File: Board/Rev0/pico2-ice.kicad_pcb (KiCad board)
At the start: 4 copper layers, 22.9 x 61 mm, 101 parts, among them J1 USB_C_Receptacle_USB2.0, J2 Conn_02x20_Odd_Even, J3 Conn_02x20_Odd_Even, J4 PB_SEL, Q1 2N7002, SW1 PTS820 J25K SMTR LFS, SW2 PTS820 J25K SMTR LFS, U1 NCP115AMX120TCG, U2 W25Q32JVSSIQ, U3 RP2040, U4 NCP115AMX330TCG, U5 APS6404L-3SQN-SN, U6 ICE40UP5K-SG48ITR, U8 W25Q32JVSSIQ, Y1 12 MHz

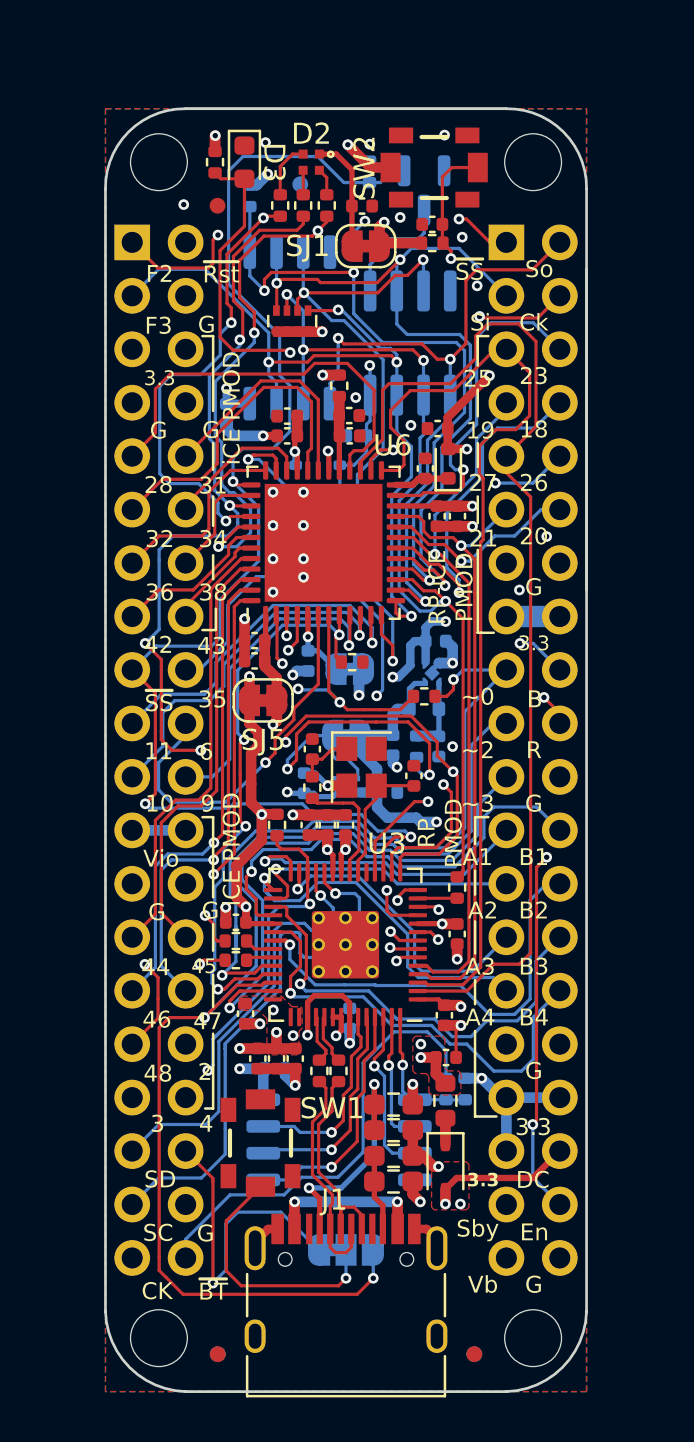
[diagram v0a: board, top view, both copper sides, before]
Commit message: Complete the layout for a review.
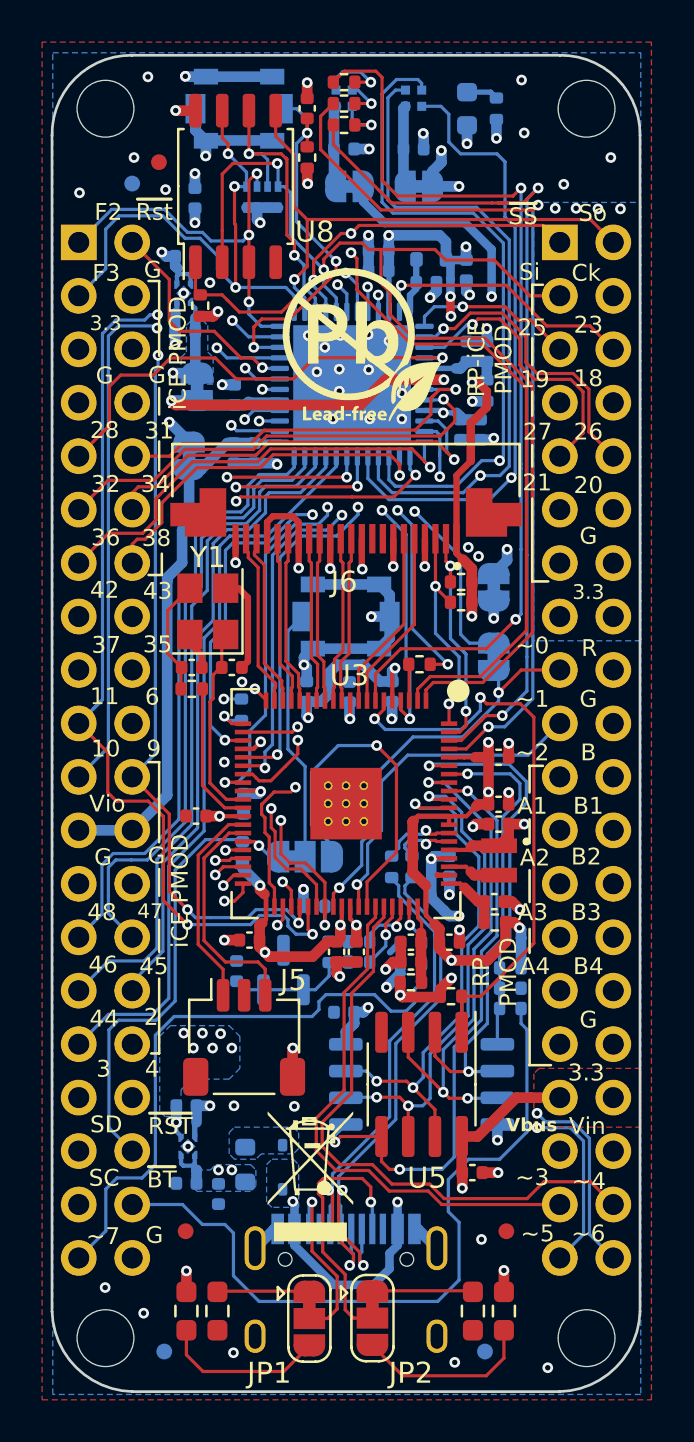
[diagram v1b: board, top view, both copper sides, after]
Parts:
- removed D6: 1N4148WT-7, Diode_SMD:D_SOD-523
- removed Q1: 2N7002, Package_TO_SOT_SMD:SOT-23
- added C20: 4.7u, Capacitor_SMD:C_0402_1005Metric, B.Cu at (77.3, 109.7)
- added C23: 4.7u, Capacitor_SMD:C_0402_1005Metric, F.Cu at (79.4, 111.3)
- added C35: 4.7u, Capacitor_SMD:C_0402_1005Metric, F.Cu at (75.5, 114.2)
- added C38: 4.7u, Capacitor_SMD:C_0402_1005Metric, F.Cu at (79.6, 107.7)
- added C39: 4.7u, Capacitor_SMD:C_0402_1005Metric, B.Cu at (64.8, 124.7)
- added C41: 4.7u, Capacitor_SMD:C_0402_1005Metric, B.Cu at (64.8, 121.0)
- added J5: SM03B-SRSS-TB, Connector_JST:JST_SH_SM03B-SRSS-TB_1x03-1MP_P1.00mm_Horizontal, F.Cu at (67.5, 117.8)
- added J6: Conn_01x22_MountingPin, RP2350_60QFN_minimal:AMPHENOL_SFV22R-2STE1HLF, F.Cu at (72.4, 91.7)
- added JP1: SolderJumper_3_Bridged12, Jumper:SolderJumper-3_P1.3mm_Bridged12_RoundedPad1.0x1.5mm, F.Cu at (70.6, 131.1)
- added JP2: SolderJumper_3_Bridged12, Jumper:SolderJumper-3_P1.3mm_Bridged12_RoundedPad1.0x1.5mm, F.Cu at (73.6, 131.1)
- added L1: 3.3u, RP2350_60QFN_minimal:L_pol_2016, F.Cu at (79.7, 109.4)
- added R26: 27, Resistor_SMD:R_0402_1005Metric, F.Cu at (79.5, 112.3)
- added R27: DNF, Resistor_SMD:R_0402_1005Metric, B.Cu at (80.2, 115.5)
- added R28: 10K, Resistor_SMD:R_0402_1005Metric, B.Cu at (75.5, 113.3)
- added R29: 10K, Resistor_SMD:R_0402_1005Metric, B.Cu at (75.5, 114.3)
- added R30: 0, Resistor_SMD:R_0402_1005Metric, B.Cu at (73.0, 114.2)
- added R31: 0, Resistor_SMD:R_0402_1005Metric, B.Cu at (73.0, 113.2)
- added SJ3: SHORT, Jumper:SolderJumper-2_P1.3mm_Bridged_RoundedPad1.0x1.5mm, B.Cu at (79.4, 99.7)
- added SJ6: SHORT, Jumper:SolderJumper-2_P1.3mm_Bridged_RoundedPad1.0x1.5mm, B.Cu at (79.4, 96.4)
- added U9: NCP115AMX330TCG, RP2040_minimal:OnSemi_XDFN4-1EP_1.0x1.0mm_EP0.52x0.52mm, B.Cu at (64.9, 123.0)
- C1, C2: value 27p -> 15p
- C15, C16, C17, C21, C22, C24, C25, C28, C29, C3, C30, C31, C32, C33, C34, C6, D1, D2, D3, D5, J1, PTC1, R11, R14, R16, R4, R5, R7, RN1, SJ1, SJ5, SW1, SW2, U6: moved to B.Cu
- C4, C42, LOGO2, LOGO3, R13, R8, U5, U8: moved to F.Cu
- C9: value 4.7u -> 0.1u; moved to F.Cu
- D4: value 1N5819WS -> MHPA1010RGBDT; footprint Diode_SMD:D_SOD-323 -> CUSTOM:LED_Cree-PLCC4_1x1mm_CW
- R12: value 27 -> 1K; moved to B.Cu
- R15: value 5.1K -> 10K; moved to F.Cu
- R20, R22: value DNI -> 56K
- R23: value 27 -> 10K
- R25: value 27 -> 100
- R3: value 10K -> DNF
- R6: value 1k -> 27
- U3: value RP2040 -> RP2350_80QFN; footprint RP2040_minimal:RP2040-QFN-56 -> RP2350_60QFN_minimal:RP2350B_QFN-80_EP_10.573x10.573_Pitch0.4mm
- U4: value NCP115AMX330TCG -> TL431DBZ; footprint RP2040_minimal:OnSemi_XDFN4-1EP_1.0x1.0mm_EP0.52x0.52mm -> Package_TO_SOT_SMD:SOT-23
- Y1: value 12 MHz -> ABM8-272-T3; footprint Crystal:Crystal_SMD_2520-4Pin_2.5x2.0mm -> Crystal:Crystal_SMD_3225-4Pin_3.2x2.5mm
- moved FID5 56.7 mm to (63.5, 76.2)
- moved FID1 50.6 mm to (80.0, 127.0)
- moved R15 36.2 mm to (77.4, 115.8)
- moved C42 35.4 mm to (78.4, 124.2), turned to 0 degrees
- moved U5 35.2 mm to (76.0, 120.0)
- moved C7 27.2 mm to (64.7, 80.7)
- moved SJ2 26.3 mm to (75.9, 77.4), turned to 0 degrees
- moved SW1 25.3 mm to (72.4, 97.8), turned to 180 degrees
- moved U1 24.6 mm to (64.7, 82.4), turned to 180 degrees
- moved C13 23.4 mm to (75.6, 75.6)
- moved C37 22.2 mm to (64.7, 84.2), turned to 180 degrees
- moved R23 20.1 mm to (77.9, 97.1), turned to 180 degrees
- moved R13 20.0 mm to (77.9, 96.1), turned to 180 degrees
- moved J4 18.8 mm to (70.4, 109.2)
- moved C11 18.3 mm to (79.6, 104.5), turned to 0 degrees
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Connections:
- C1 pad 1: /XIN -> Net-(C1-Pad1)
- C13 pad 1: +3V3 -> Net-(D4-A)
- C2 pad 1: Net-(C2-Pad1) -> /XIN
- C21 pad 1: +3V3 -> +3V3_FPGA
- C22 pad 1: +3V3 -> +3V3_FPGA
- C24 pad 1: +3V3 -> +3V3_FPGA
- C25 pad 1: +3V3 -> +3V3_FPGA
- C26 pad 1: +3V3 -> +3V3_FPGA
- C28 pad 1: +3V3 -> +3V3_FPGA
- C3 pad 1: VBUS -> V_{in}
- C36 pad 1: Net-(D6-A) -> Net-(U4-K)
- C42 pad 1: /+3V3_STDBY -> +3V3
- C7 pad 1: VBUS -> +3V3_FPGA
- C9 pad 1: VBUS -> Net-(U3-ADC_AVDD)
- D1 pad 2: +3V3 -> +3V3_FPGA
- D4 pad 1: /+3V3_STDBY -> Net-(D4-A)
- D4 pad 2: +3V3 -> /ICE_LED_R
- D5 pad 2: VDC -> V_{BUS}
- J1 pad A4: VDC -> V_{BUS}
- J1 pad A9: VDC -> V_{BUS}
- J1 pad B4: VDC -> V_{BUS}
- J1 pad B9: VDC -> V_{BUS}
- J2 pad 1: /ICE_FLASH_IO2 -> /ICE_12|IO2
- J2 pad 17: /SRAM_SS -> /ICE_37
- J2 pad 27: /ICE_44_G6 -> /ICE_48
- J2 pad 28: /ICE_45 -> /ICE_47
- J2 pad 3: /ICE_FLASH_IO3 -> /ICE_13|IO3
- J2 pad 30: /ICE_47 -> /ICE_45
- J2 pad 31: /ICE_48 -> /ICE_44_G6
- J2 pad 35: /SWD -> /SDA_GPIO2
- J2 pad 37: /SWCLK -> /SCL_GPIO3
- J2 pad 38: GND -> /~{USB_BOOT}
- J2 pad 39: /PICO_CLKOUT -> /ADC7
- J2 pad 40: /~{USB_BOOT} -> GND
- J2 pad 5: +3V3 -> +3V3_FPGA
- J2 pad 6: +3V3 -> +3V3_FPGA
- J3 pad 15: +3V3 -> +3V3_FPGA
- J3 pad 16: +3V3 -> +3V3_FPGA
- J3 pad 17: /ICE_DONE_ADC0 -> /ICE_DONE|ADC0
- J3 pad 18: /LED_B -> /ICE_LED_R
- J3 pad 19: /ADC2|PB -> /ADC1
- J3 pad 20: /LED_R -> /ICE_LED_G
- J3 pad 21: /ADC3 -> /ADC2|PB
- J3 pad 22: /LED_G -> /ICE_LED_B
- J3 pad 35: +3V3 -> V_{BUS}
- J3 pad 36: VDC -> V_{in}
- J3 pad 37: /+3V3_STDBY -> /ADC3
- J3 pad 38: /PWR_EN -> /ADC4
- J3 pad 39: VBUS -> /ADC5|VREF
- J3 pad 40: GND -> /ADC6
- PTC1 pad 1: VBUS -> V_{in}
- R1 pad 2: Net-(C2-Pad1) -> Net-(C1-Pad1)
- R10 pad 1: Net-(J1-CC1) -> Net-(JP2-A)
- R12 pad 1: /ICE_35_G0 -> Net-(R12-Pad1)
- R12 pad 2: /ICE_CLK -> Net-(U4-K)
- R13 pad 1: GND -> +3V3
- R13 pad 2: /SRAM_SS -> /SDA_GPIO2
- R14 pad 2: +3V3 -> +3V3_FPGA
- R15 pad 1: /+3V3_STDBY -> +3V3
- R15 pad 2: Net-(Q1-D) -> /~{SRAM_SS}
- R2 pad 1: /QSPI_SS -> /~{QSPI_SS}
- R20 pad 1: VDC -> V_{BUS}
- R20 pad 2: Net-(J1-CC2) -> Net-(JP1-B)
- R21 pad 1: +3V3 -> +3V3_FPGA
- R22 pad 1: VDC -> V_{BUS}
- R22 pad 2: Net-(J1-CC1) -> Net-(JP2-B)
- R23 pad 1: /PICO_CLKOUT -> +3V3
- R23 pad 2: Net-(U3-GPIO25) -> /SCL_GPIO3
- R24 pad 1: Net-(J1-CC2) -> Net-(JP1-A)
- R25 pad 1: /ICE_DONE -> Net-(U3-ADC_AVDD)
- R25 pad 2: /ICE_DONE_ADC0 -> +3V3
- R3 pad 2: /QSPI_SS -> /~{QSPI_SS}
- R6 pad 1: /PWR_EN -> /ICE_35_G0
- R6 pad 2: Net-(D6-A) -> Net-(U3-GPIO21)
- R8 pad 2: +3V3 -> +3V3_FPGA
- R9 pad 2: Net-(U3-GPIO10) -> Net-(U3-GPIO6)
- RN1 pad 5: /ICE_FLASH_IO3 -> /ICE_13|IO3
- RN1 pad 6: /ICE_FLASH_IO2 -> /ICE_12|IO2
- SJ2 pad 1: VBUS -> Net-(D4-A)
- SJ2 pad 2: /PWR_EN -> +3V3_FPGA
- SJ5 pad 1: +3V3 -> +3V3_FPGA
- U1 pad 3: /PWR_EN -> +3V3_FPGA
- U1 pad 4: VBUS -> +3V3_FPGA
- U2 pad 1: /QSPI_SS -> /~{QSPI_SS}
- U3 pad 1: +3V3 -> /ICE_SI
- U3 pad 10: +3V3 -> +1V1
- U3 pad 11: /ICE_SI -> /Lane2_N
- U3 pad 12: /ICE_SSN -> /Lane2_P
- U3 pad 13: Net-(U3-GPIO10) -> /Clock_P
- U3 pad 14: /ICE_SO -> /Clock_N
- U3 pad 15: /LED_G -> +3V3
- U3 pad 16: /LED_R -> /Lane1_P
- U3 pad 17: /SRAM_SS -> /Lane1_N
- U3 pad 18: /LED_B -> /Lane0_P
- U3 pad 19: GND -> /Lane0_N
- U3 pad 2: /ICE_27 -> /ICE_SSN
- U3 pad 20: /XIN -> /ICE_27
- U3 pad 21: /XOUT -> Net-(U3-GPIO21)
- U3 pad 22: +3V3 -> /ICE_21
- U3 pad 23: +1V1 -> /ICE_19
- U3 pad 24: /SWCLK -> +3V3
- U3 pad 25: /SWD -> /ICE_26
- U3 pad 26: /~{RESET} -> /ICE_23
- U3 pad 27: /PICO_PMOD_A3 -> /ICE_20_G3
- U3 pad 28: /PICO_PMOD_A1 -> /ICE_18
- U3 pad 29: /PICO_PMOD_A4 -> +3V3
- U3 pad 3: /ICE_25 -> Net-(U3-GPIO6)
- U3 pad 30: /PICO_PMOD_A2 -> /XIN
- U3 pad 31: /PICO_PMOD_B3 -> /XOUT
- U3 pad 32: /PICO_PMOD_B1 -> +1V1
- U3 pad 33: +3V3 -> /SWCLK
- U3 pad 34: /PICO_PMOD_B4 -> /SWD
- U3 pad 35: /PICO_PMOD_B2 -> /~{RESET}
- U3 pad 36: /ICE_CLK -> /PICO_PMOD_A3
- U3 pad 37: Net-(U3-GPIO25) -> /PICO_PMOD_A1
- U3 pad 38: /ICE_DONE_ADC0 -> /PICO_PMOD_A4
- U3 pad 39: /~{ICE_RST} -> /PICO_PMOD_A2
- U3 pad 4: /ICE_21 -> /ICE_SO
- U3 pad 40: /ADC2|PB -> /PICO_PMOD_B3
- U3 pad 41: /ADC3 -> +3V3
- U3 pad 42: +3V3 -> /PICO_PMOD_B1
- U3 pad 43: +3V3 -> /PICO_PMOD_B4
- U3 pad 44: +3V3 -> /PICO_PMOD_B2
- U3 pad 45: +1V1 -> /ICE_9
- U3 pad 46: /USB_N -> /ICE_11
- U3 pad 47: /USB_P -> /ICE_25
- U3 pad 48: +3V3 -> /~{ICE_RST}
- U3 pad 49: +3V3 -> /ICE_DONE|ADC0
- U3 pad 5: /ICE_19 -> +3V3
- U3 pad 50: +1V1 -> +3V3
- U3 pad 51: /QSPI_SD3 -> +1V1
- U3 pad 52: /QSPI_SCLK -> /ADC1
- U3 pad 53: /QSPI_SD0 -> /ADC2|PB
- U3 pad 54: /QSPI_SD2 -> /ADC3
- U3 pad 55: /QSPI_SD1 -> /ADC4
- U3 pad 56: /QSPI_SS -> /ADC5|VREF
- U3 pad 57: GND -> /ADC6
- U3 pad 6: /ICE_26 -> /~{SRAM_SS}
- U3 pad 7: /ICE_23 -> /LED_B
- U3 pad 8: /ICE_20_G3 -> /GPIO10
- U3 pad 9: /ICE_18 -> /GPIO11
- U4 pad 1: +3V3 -> Net-(U4-K)
- U4 pad 2: GND -> Net-(U4-K)
- U4 pad 3: Net-(D6-A) -> GND
- U5 pad 1: Net-(Q1-D) -> /~{SRAM_SS}
- U5 pad 2: /ICE_SI -> /QSPI_SD1
- U5 pad 3: /ICE_FLASH_IO2 -> /QSPI_SD2
- U5 pad 5: /ICE_SO -> /QSPI_SD0
- U5 pad 6: /ICE_SCK -> /QSPI_SCLK
- U5 pad 7: /ICE_FLASH_IO3 -> /QSPI_SD3
- U5 pad 8: /+3V3_STDBY -> +3V3
- U6 pad 12: /ICE_FLASH_IO2 -> /ICE_12|IO2
- U6 pad 13: /ICE_FLASH_IO3 -> /ICE_13|IO3
- U6 pad 22: +3V3 -> +3V3_FPGA
- U6 pad 33: +3V3 -> +3V3_FPGA
- U6 pad 37: /SRAM_SS -> /ICE_37
- U6 pad 39: /LED_G -> /ICE_LED_G
- U6 pad 40: /LED_B -> /ICE_LED_B
- U6 pad 41: /LED_R -> /ICE_LED_R
- U6 pad 7: /ICE_DONE -> Net-(U6B-CDONE)
- U8 pad 3: /ICE_FLASH_IO2 -> /ICE_12|IO2
- U8 pad 7: /ICE_FLASH_IO3 -> /ICE_13|IO3
- U8 pad 8: +3V3 -> +3V3_FPGA
- Y1 pad 1: Net-(C2-Pad1) -> /XIN
- Y1 pad 3: /XIN -> Net-(C1-Pad1)
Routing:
- net /+3V3_STDBY: track 78.0 -> 0.00 mm, vias 3 -> 0
- net /SRAM_SS: track 64.9 -> 0.00 mm, vias 3 -> 0
- net /ICE_LED_B: track 0.00 -> 49.0 mm, vias 0 -> 1
- net /SCL_GPIO3: track 0.00 -> 48.9 mm, vias 0 -> 2
- net /SDA_GPIO2: track 0.00 -> 48.5 mm, vias 0 -> 2
- net /ICE_LED_G: track 0.00 -> 47.7 mm, vias 0 -> 1
- net /ICE_FLASH_IO2: track 44.8 -> 0.00 mm, vias 4 -> 0
- net /PWR_EN: track 43.2 -> 0.00 mm, vias 4 -> 0
- net /ICE_LED_R: track 0.00 -> 42.3 mm, vias 0 -> 1
- net GND: track 34.6 -> 76.8 mm, vias 37 -> 73
- net /ICE_DONE: track 40.7 -> 1.51 mm, vias 3 -> 0
- net /ICE_FLASH_IO3: track 38.1 -> 0.00 mm, vias 4 -> 0
- net /ICE_DONE_ADC0: track 35.1 -> 0.00 mm, vias 2 -> 0
- net /ICE_11: track 16.8 -> 49.6 mm, vias 1 -> 4
- net /ADC2|PB: track 58.6 -> 26.2 mm, vias 2 -> 1
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- added copper zone on In1.Cu, net +1V1
- added copper zone on B.Cu, net +1V2
- added copper zone on B.Cu, net +3V3
- added copper zone on B.Cu, net +3V3_FPGA
- added copper zone on In2.Cu, net +3V3_FPGA
- added copper zone on B.Cu, net Net-(D5-K)
- added copper zone on B.Cu, net V_{BUS}
- added copper zone on In2.Cu, net V_{BUS}
- added copper zone on B.Cu, net V_{in}
- added copper zone on In2.Cu, net V_{in}
- removed copper zone on F.Cu, net VBUS
- removed copper zone on In2.Cu, net VBUS
- removed copper zone on F.Cu, net VDC
- removed copper zone on In2.Cu, net VDC
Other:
- board size 22.9 x 61 mm -> 27.9 x 63.5 mm
- board text added: "37"
- board text added: "Vbus"
- board text added: "Vin"
- board text added: "pico-ice"
- board text added: "rev3"
- board text added: "~1"
- board text added: "~4"
- board text added: "~5"
- board text added: "~6"
- board text added: "~7"
- board text added: "~{RST}"
- board text removed: "CK"
- board text removed: "DC"
- board text removed: "En"
- board text removed: "Sby"
- board text removed: "Vb"
- board text removed: "pico-ice Rev3"
